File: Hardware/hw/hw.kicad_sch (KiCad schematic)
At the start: 14 parts, among them Q1 FS8205A, U1 ESP32-C6-WROOM-1, U2 RV-3028-C7, U4 SC189LSKTRT, U5 TP4056-42-ESOP8, U6 TPS63002DRCT

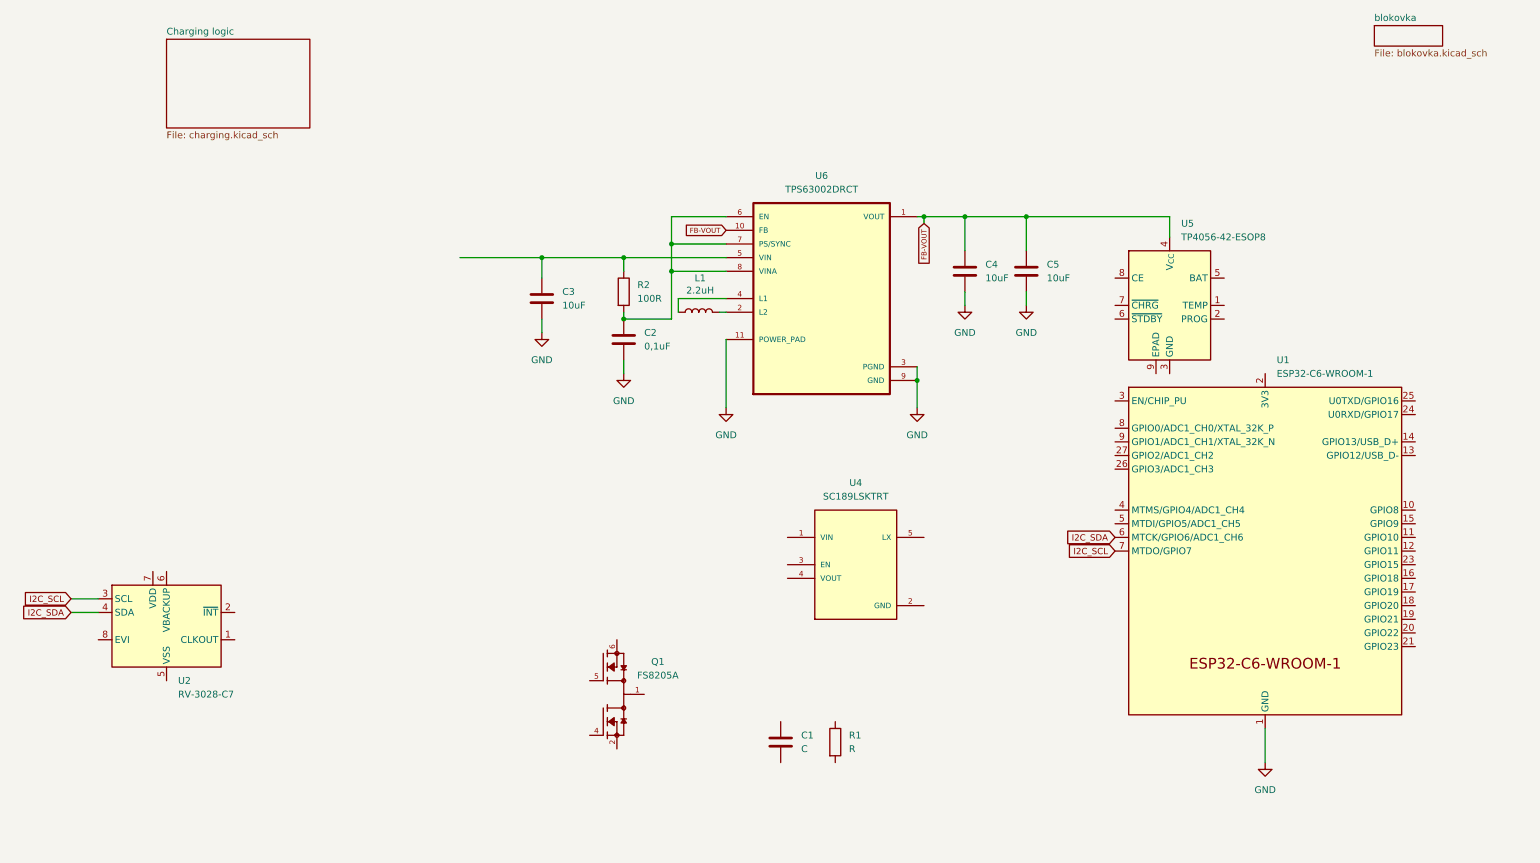
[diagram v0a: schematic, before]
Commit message: IoT board update
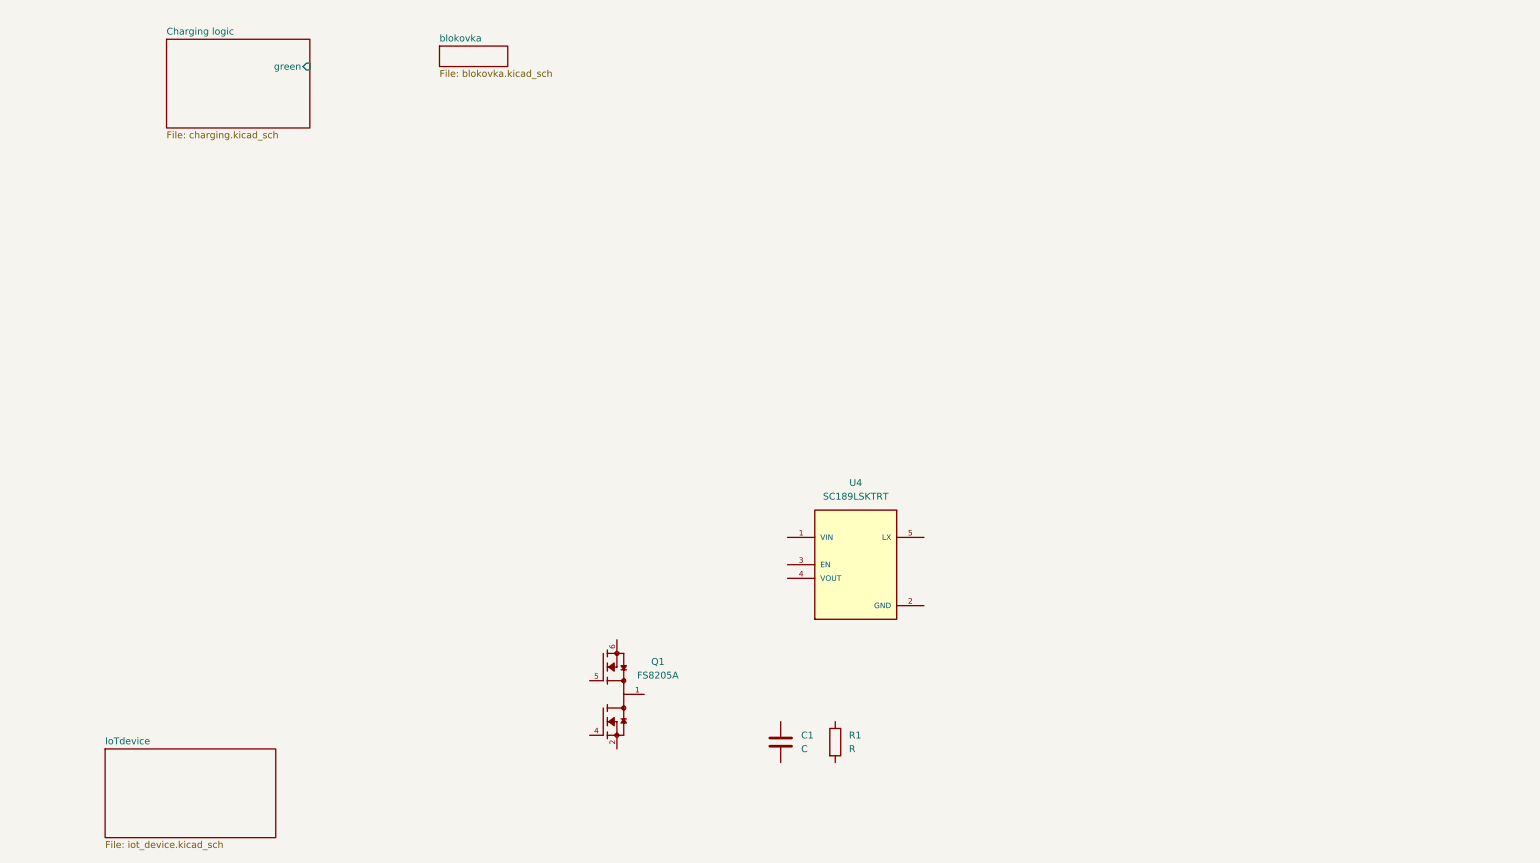
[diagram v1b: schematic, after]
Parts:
- removed C2: 0,1uF, Capacitor_SMD:C_0805_2012Metric, symbol Device:C
- removed C3, C4, C5: 10uF, Capacitor_SMD:C_0805_2012Metric, symbol Device:C
- removed L1: 2.2uH, Inductor_SMD:L_0201_0603Metric, symbol Device:L
- removed R2: 100R, Resistor_SMD:R_0805_2012Metric, symbol Device:R
- removed U1: ESP32-C6-WROOM-1, PCM_Espressif:ESP32-C6-WROOM-1, symbol PCM_Espressif:ESP32-C6-WROOM-1
- removed U2: RV-3028-C7, Package_SON:MicroCrystal_C7_SON-8_1.5x3.2mm_P0.9mm, symbol Timer_RTC:RV-3028-C7
- removed U5: TP4056-42-ESOP8, Package_SO:SOIC-8-1EP_3.9x4.9mm_P1.27mm_EP2.41x3.3mm_ThermalVias, symbol Battery_Management:TP4056-42-ESOP8
- removed U6: TPS63002DRCT, TPS63002DRCT:VREG_V62_16624-01YE, symbol TPS63002DRCT:TPS63002DRCT
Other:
- added sheet IoTdevice (iot_device.kicad_sch)
- sheet Charging logic ports: added green; removed none
